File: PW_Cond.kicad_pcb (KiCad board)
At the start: 2 copper layers, 38 x 33 mm, 25 parts, among them J1 Conn_01x02_Female, J2 Conn_01x04_Female, J3 Conn_01x02_Female, Q1 BC847, U1 MCP602, U2 MCP602

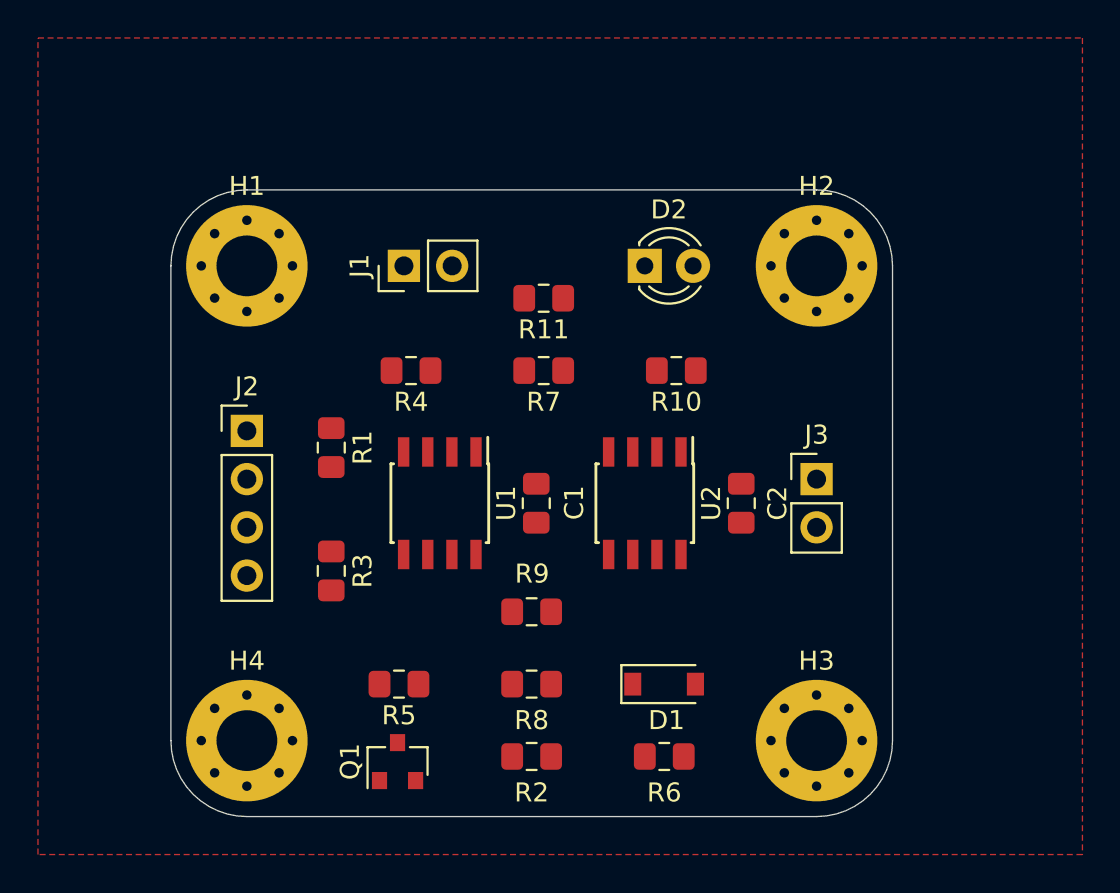
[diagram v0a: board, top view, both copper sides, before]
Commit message: board v1 finished
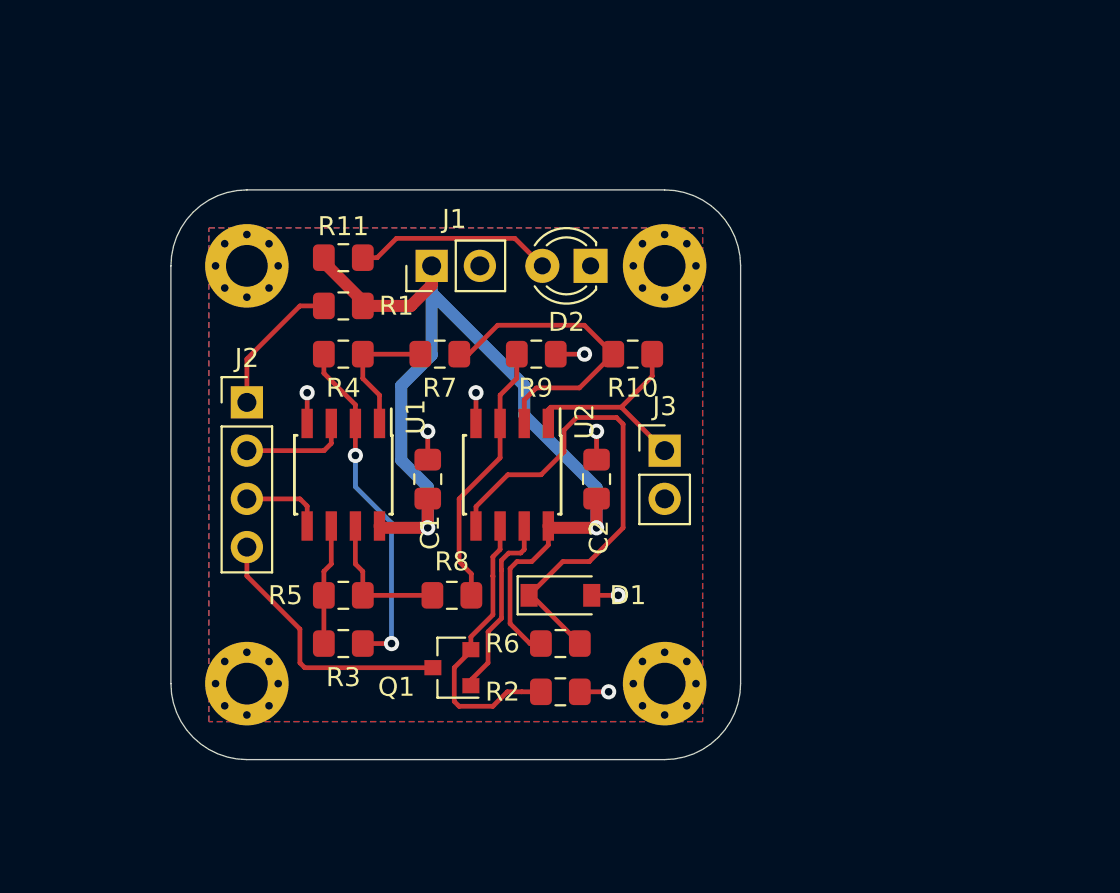
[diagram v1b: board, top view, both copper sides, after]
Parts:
- H1, H2, H3, H4: footprint MountingHole:MountingHole_3.2mm_M3_Pad_Via -> MountingHole:MountingHole_2.2mm_M2_Pad_Via
- moved R9 13.6 mm to (115.2, 104.7), turned to 0 degrees
- moved R11 10.8 mm to (105.1, 99.6), turned to 0 degrees
- moved H3 8.54 mm to (122.0, 122.0)
- moved J3 8.14 mm to (122.0, 109.7)
- moved R6 8.08 mm to (116.5, 119.9), turned to 0 degrees
- moved H2 8.00 mm to (122.0, 100.0)
- moved C2 7.73 mm to (118.4, 111.2)
- moved R1 7.49 mm to (105.1, 102.1), turned to 180 degrees
- moved D1 7.19 mm to (116.5, 117.3)
- moved U2 7.14 mm to (114.0, 111.0)
- moved R8 6.28 mm to (110.8, 117.3)
- moved C1 5.85 mm to (109.5, 111.2)
- moved Q1 5.71 mm to (110.8, 121.2), turned to 180 degrees
- moved R7 5.54 mm to (110.2, 104.7)
- moved R5 5.52 mm to (105.1, 117.3)
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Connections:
- D2 pad 1: Net-(D2-Pad1) -> GND
- D2 pad 2: +15V -> Net-(D2-Pad2)
- R11 pad 1: Net-(D2-Pad1) -> +15V
- R11 pad 2: GND -> Net-(D2-Pad2)
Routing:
- net +15V: track 0.00 -> 56.7 mm, vias 0 -> 2
- net Net-(D1-Pad1): track 0.00 -> 27.1 mm
- net Net-(R3-Pad1): track 0.00 -> 18.2 mm, vias 0 -> 2
- net Net-(R10-Pad2): track 0.00 -> 16.3 mm
- net Net-(Q1-Pad2): track 0.00 -> 15.2 mm
- net /MAP: track 0.00 -> 14.4 mm
- net Net-(R8-Pad1): track 0.00 -> 14.2 mm
- net /Meusure: track 0.00 -> 11.3 mm
- net GND: track 0.00 -> 10.6 mm, vias 0 -> 7
- net Net-(D2-Pad2): track 0.00 -> 10.5 mm
- net Net-(Q1-Pad1): track 0.00 -> 9.95 mm
- net /PAP: track 0.00 -> 7.50 mm
- net Net-(R5-Pad1): track 0.00 -> 7.48 mm
- net Net-(R4-Pad1): track 0.00 -> 7.04 mm
- net Net-(R3-Pad2): track 0.00 -> 6.35 mm
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- added copper zone on B.Cu, net GND
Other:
- board size 38 x 33 mm -> 30 x 30 mm
